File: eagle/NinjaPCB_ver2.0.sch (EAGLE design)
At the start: 76 parts, among them IC2 VNH3SP30-BNC, IC3 ANALOGSW_AD_SOT23-6NC, IC4 ANALOGSW_TI-SC70-5/6NC, IC5 MCP3551SNNC, IC6 NAU7802NC, J2 ATX24, J3 HEATER, J4 HEATER_TEMP, J5 PELTIER, Q2 IRF520NPBF, Q3 IRF520NPBF, U1 CJT1117-3.3-SOT223

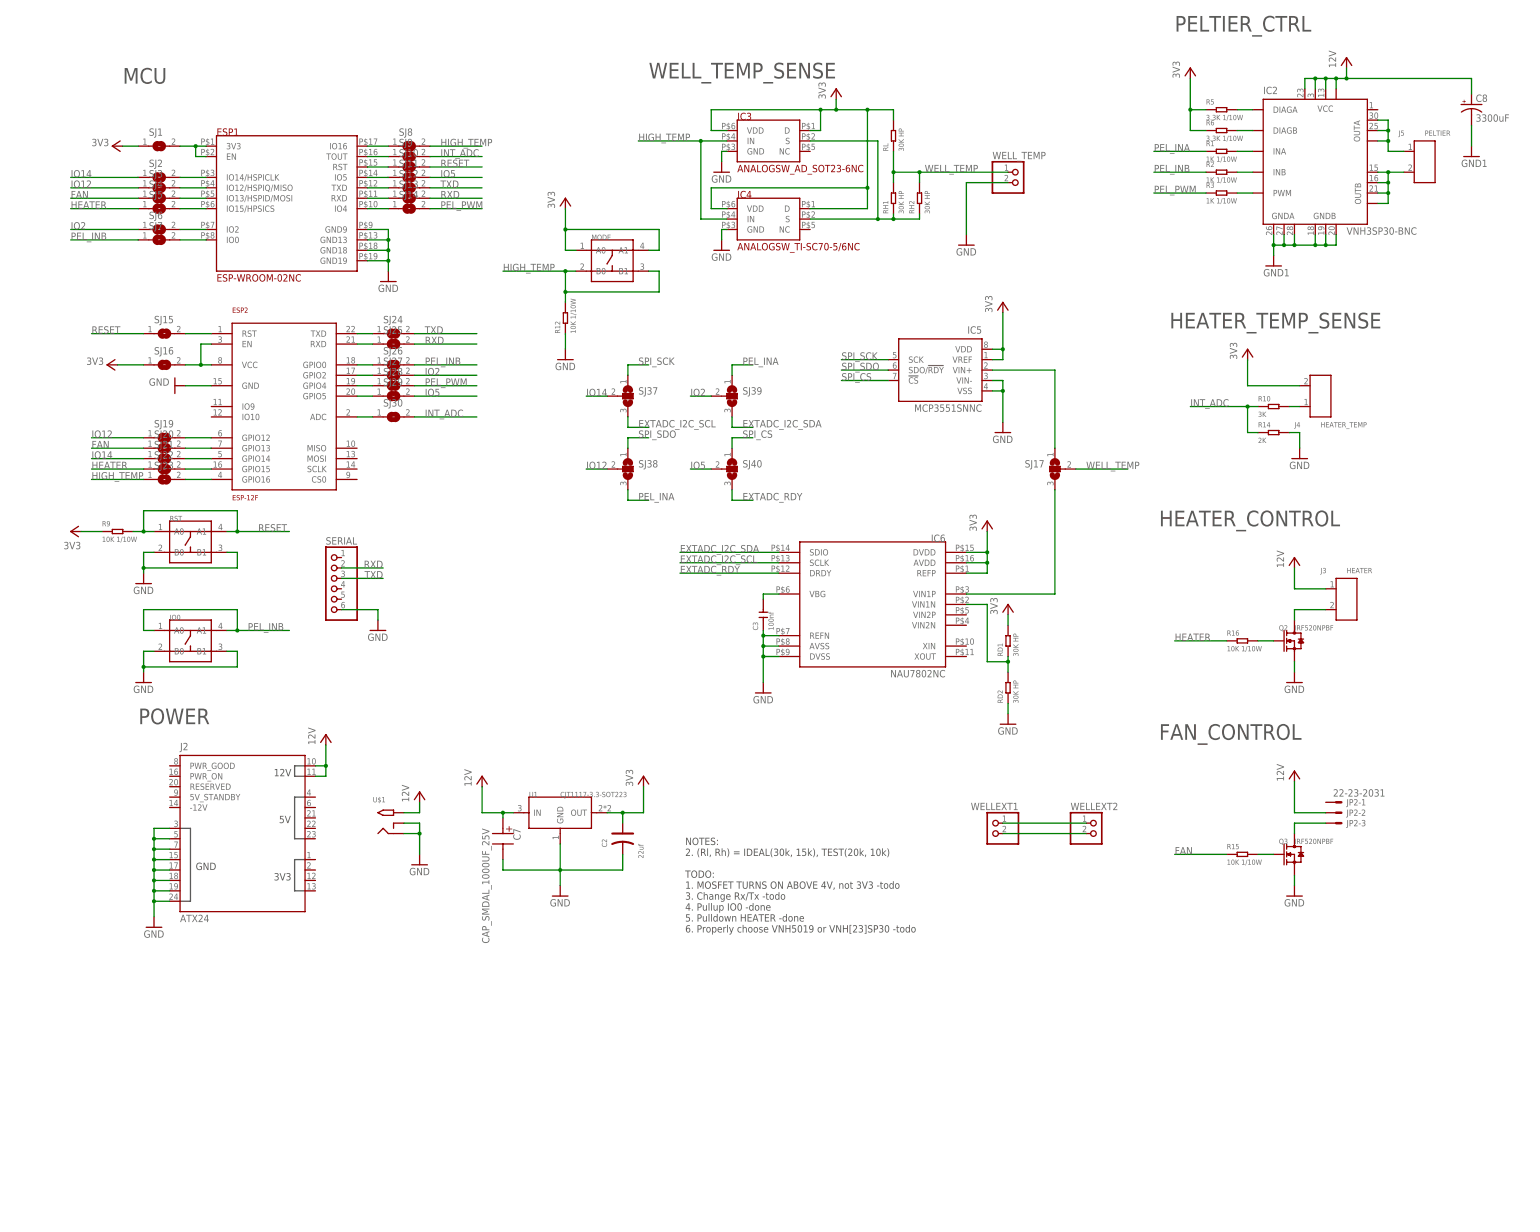
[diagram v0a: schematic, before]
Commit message: set default 4x4
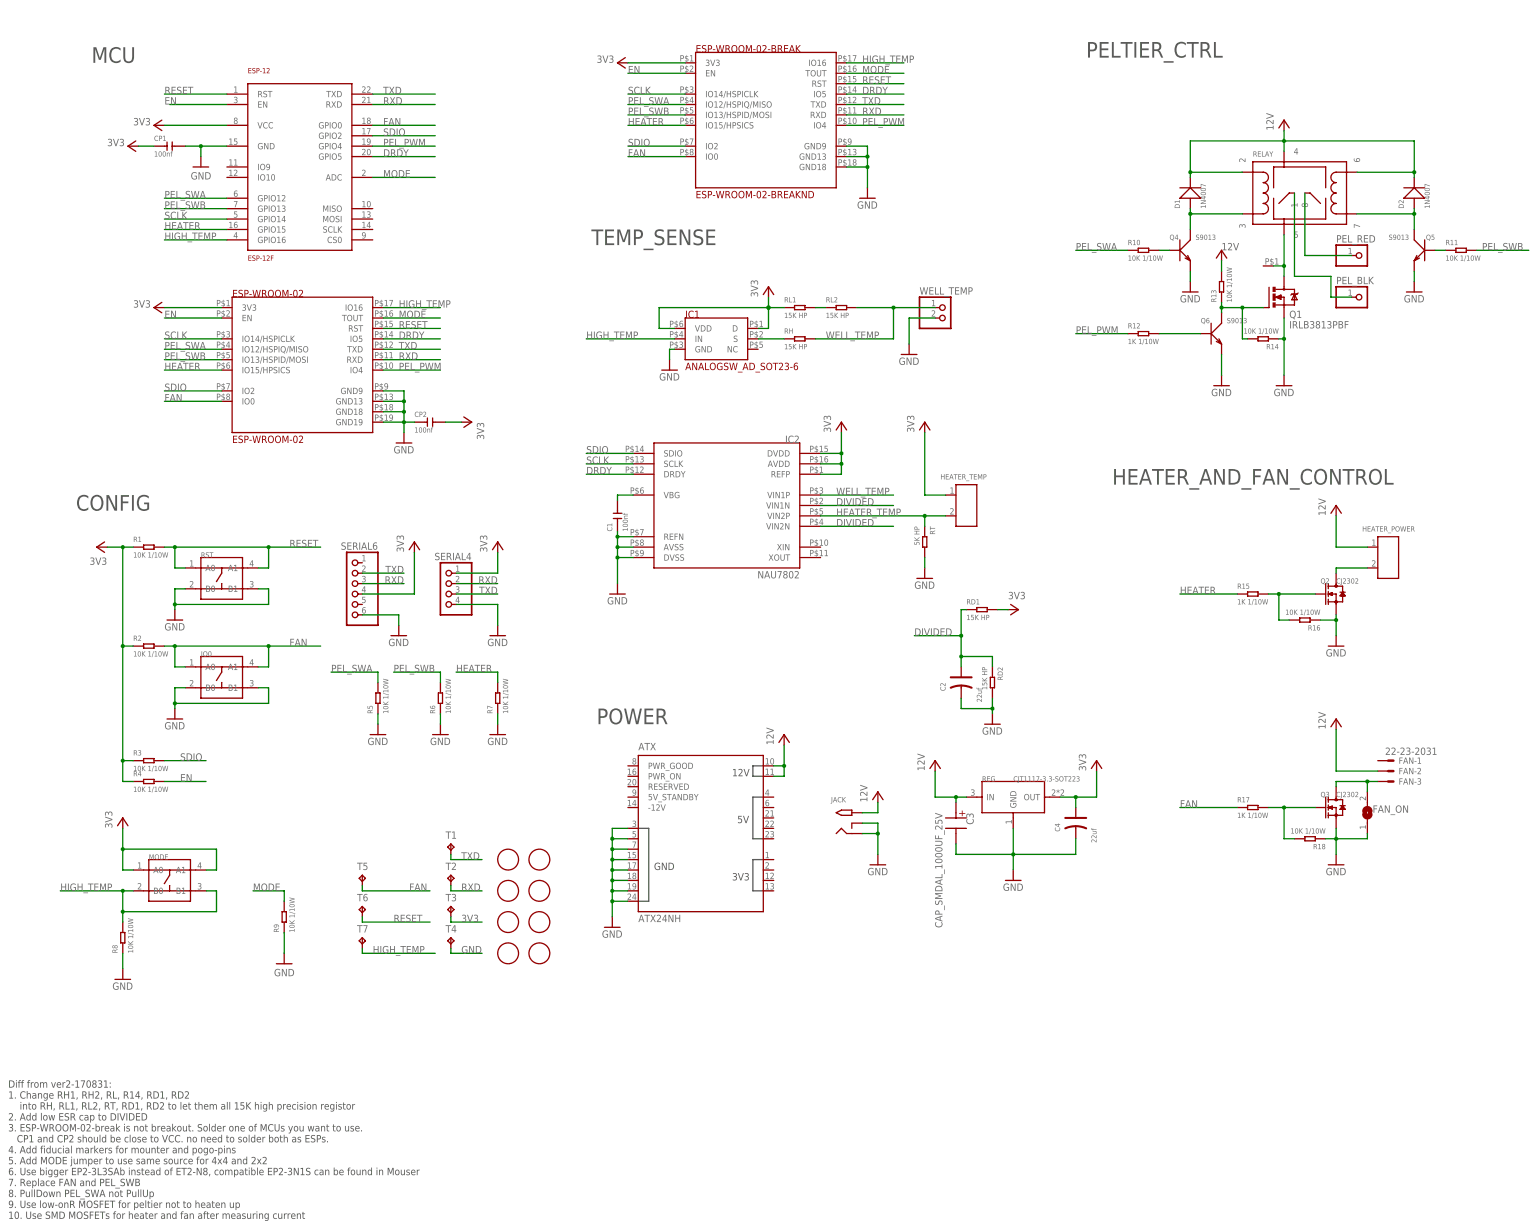
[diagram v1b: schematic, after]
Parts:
- removed C7: CAP_SMDAL_1000UF_25V, Seeed-OPL-2017-01-Capacitor-akita:CAP_SMDAL_1000UF_25V
- removed C8: 3300uF, PCR-RCL:CAP_E5-13-L3030RINV
- removed ESP1: ESP-WROOM-02NC, PCR-Module:ESP-WROOM-02NC
- removed ESP2: ESP-12F, Seeed-OPL-2017-01-Sensor-camilo:ESP-12F
- removed IC3: ANALOGSW_AD_SOT23-6NC, PCR-IC:ANALOGSW_AD_SOT23-6NC
- removed IC4: ANALOGSW_TI-SC70-5/6NC, PCR-IC:ANALOGSW_TI-SC70-5/6NC
- removed IC5: MCP3551SNNC, microchip:MCP3551SNNC
- removed IC6: NAU7802NC, PCR-IC:NAU7802NC
- removed J2: ATX24, PCR-Connector:ATX24
- removed J3: HEATER, Seeed-Connector:SCREW-TERMINAL-GREEN(2P-3.5)
- removed J4: HEATER_TEMP, Seeed-Connector:SCREW-TERMINAL-GREEN(2P-3.5)
- removed J5: PELTIER, Seeed-Connector:SCREW-TERMINAL-GREEN(2P-3.5)
- removed JP2: 22-23-2031, con-molex:22-23-2031
- removed RH1, RH2, RL: 30K HP, PCR-RCL:R0603NC
- removed SERIAL: (no value), pinhead:PINHD-1X6
- removed SJ1, SJ10, SJ11, SJ12, SJ13, SJ14, SJ15, SJ16, SJ19, SJ2, SJ20, SJ21, SJ22, SJ23, SJ24, SJ25, SJ26, SJ27, SJ28, SJ29, SJ3, SJ30, SJ4, SJ5, SJ6, SJ7, SJ8, SJ9: (no value), jumper:SJ
- removed SJ17, SJ37, SJ38, SJ39, SJ40: (no value), jumper:SJ2W
- removed U$1: 2.1MMJACKTHM, adafruit:2.1MMJACKTHM
- removed U1: CJT1117-3.3-SOT223, Seeed-IC:PMIC-CJT1117-3.3(SOT223)
- removed WELLEXT1, WELLEXT2: (no value), pinhead:PINHD-1X2
- added ATX: ATX24NH, PCR-Connector:ATX24NH
- added C1, CP1, CP2: 100nf, Seeed-Capacitor:CERAMIC-100NF-50V-10%-X7R(0603)
- added C4: 22uf, Seeed-Capacitor:TANTALUM-SMD-22UF-16V(AVX-B)
- added D1, D2: 1N4007, Seeed-Diode:DIODE-GEN-PURPOSE-1KV-1A(DO-214AC)
- added ESP-12: ESP-12F, Seeed-OPL-2017-01-Sensor-camilo:ESP-12F
- added ESP-WROOM-02: ESP-WROOM-02, PCR-Module:ESP-WROOM-02
- added ESP-WROOM-02-BREAK: ESP-WROOM-02-BREAKND, PCR-Module:ESP-WROOM-02-BREAKND
- added FAN: 22-23-2031, con-molex:22-23-2031
- added FAN_ON: (no value), jumper:SJ
- added HEATER_POWER, HEATER_TEMP: (no value), Seeed-Connector:SCREW-TERMINAL-GREEN(2P-3.5)
- added HEATSINK: HEAT111PB015, PCR-Connector:HEAT111PB015
- added IC1: ANALOGSW_AD_SOT23-6, PCR-IC:ANALOGSW_AD_SOT23-6
- added JACK: 2.1MMJACKTHM-NOOUT, adafruit:2.1MMJACKTHM-NOOUT
- added PEL_BLK, PEL_RED: (no value), pinhead:PINHD-1X1L
- added Q1: IRLB3813PBF, transistor-power:IRF520
- added Q4, Q5, Q6: S9013, Seeed-Transistor:SMD-TRANSISTORS-NPN-25V-500MA-S9013(SOT-23)
- added R11, R13, R18, R4, R7, R8: 10K 1/10W, Seeed-Resistor:SMD-RES-10K-5%-1/10W(0603)
- added R17: 1K 1/10W, Seeed-Resistor:SMD-RES-1K-5%-1/10W(0603)
- added REG: CJT1117-3.3-SOT223, Seeed-IC:PMIC-CJT1117-3.3(SOT223)
- added RELAY: NEC-RELAY2EP2, PCR-Switch:NEC-RELAY2EP2
- added RH, RL1, RL2: 15K HP, PCR-RCL:R0603
- added RT: 5K HP, Seeed-Resistor:SMD-RES-2K-1%-1/10W(0603)
- added SERIAL4: (no value), pinhead:PINHD-1X4
- added SERIAL6: (no value), pinhead:PINHD-1X6
- added T1, T2, T3, T4, T5, T6, T7: TPTP20R, testpad:TPTP20R
- added U$10, U$3, U$4, U$5, U$6, U$7, U$8, U$9: FIDUCIAL, adafruit:FIDUCIAL
- C3: value 100nf -> CAP_SMDAL_1000UF_25V; device Seeed-Capacitor:CERAMIC-100NF-50V-10%-X7R(0603) -> Seeed-OPL-2017-01-Capacitor-akita:CAP_SMDAL_1000UF_25V
- IC2: value VNH3SP30-BNC -> NAU7802; device st-microelectronics:VNH3SP30-BNC -> PCR-IC:NAU7802
- Q2, Q3: value IRF520NPBF -> CJ2302; device Seeed-Transistor:DIP-MOSFET-N-CH-100V-9.7A-IRF520NPBF(TO-220AB) -> Seeed-Transistor:SMD-MOSFET-N-CH-20V-2.1A-CJ2302(SOT-23)
- R1, R2, R3: value 1K 1/10W -> 10K 1/10W; device Seeed-Resistor:SMD-RES-1K-5%-1/10W(0603) -> Seeed-Resistor:SMD-RES-10K-5%-1/10W(0603)
- R10: value 3K -> 10K 1/10W; device Seeed-Resistor:SMD-RES-3K-1%-1/10W(0603) -> Seeed-Resistor:SMD-RES-10K-5%-1/10W(0603)
- R12, R15: value 10K 1/10W -> 1K 1/10W; device Seeed-Resistor:SMD-RES-10K-5%-1/10W(0603) -> Seeed-Resistor:SMD-RES-1K-5%-1/10W(0603)
- R14: value 2K -> 10K 1/10W; device Seeed-Resistor:SMD-RES-2K-1%-1/10W(0603) -> Seeed-Resistor:SMD-RES-10K-5%-1/10W(0603)
- R5, R6: value 3.3K 1/10W -> 10K 1/10W; device Seeed-Resistor:SMD-RES-3.3K-5%-1/10W(0603) -> Seeed-Resistor:SMD-RES-10K-5%-1/10W(0603)
- RD1, RD2: value 30K HP -> 15K HP; device PCR-RCL:R0603NC -> PCR-RCL:R0603
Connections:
- removed net EXTADC_I2C_SCL: IC6.SCLK, SJ37.3
- removed net EXTADC_I2C_SDA: IC6.SDIO, SJ39.3
- removed net EXTADC_RDY: IC6.DRDY, SJ40.3
- removed net I2C_WELL_TEMP: IC6.VIN1P, SJ17.3
- removed net INT_ADC: R10.1, R14.1, SJ30.2, SJ9.2
- removed net IO12: SJ19.1, SJ3.1, SJ38.2
- removed net IO14: SJ2.1, SJ21.1, SJ37.2
- removed net IO2: SJ27.2, SJ39.2, SJ6.1
- removed net IO5: SJ11.2, SJ29.2, SJ40.2
- removed net N$10: IC2.PWM, R3.2
- removed net N$11: ESP1.3V3, ESP1.EN, SJ1.2
- removed net N$12: ESP1.IO14/HSPICLK, SJ2.2
- removed net N$13: ESP1.IO12/HSPIQ/MISO, SJ3.2
- removed net N$14: ESP1.IO13/HSPID/MOSI, SJ4.2
- removed net N$15: ESP1.IO15/HPSICS, SJ5.2
- removed net N$16: ESP1.IO2, SJ6.2
- removed net N$17: ESP1.IO0, SJ7.2
- removed net N$18: ESP1.IO16, SJ8.1
- removed net N$19: ESP1.TOUT, SJ9.1
- removed net N$20: ESP1.RST, SJ10.1
- removed net N$21: ESP1.IO5, SJ11.1
- removed net N$22: ESP1.TXD, SJ12.1
- removed net N$23: ESP1.RXD, SJ13.1
- removed net N$24: ESP1.IO4, SJ14.1
- removed net N$26: WELLEXT1.1, WELLEXT2.1
- removed net N$28: WELLEXT1.2, WELLEXT2.2
- removed net N$40: ESP2.RST, SJ15.2
- removed net N$42: ESP2.EN, ESP2.VCC, SJ16.2
- removed net N$43: ESP2.TXD, SJ24.1
- removed net N$44: ESP2.RXD, SJ25.1
- removed net N$45: ESP2.GPIO0, SJ26.1
- removed net N$46: ESP2.GPIO2, SJ27.1
- removed net N$47: ESP2.GPIO4, SJ28.1
- removed net N$48: ESP2.GPIO5, SJ29.1
- removed net N$49: ESP2.ADC, SJ30.1
- removed net N$67: ESP2.GPIO12, SJ19.2
- removed net N$68: ESP2.GPIO13, SJ20.2
- removed net N$69: ESP2.GPIO14, SJ21.2
- removed net N$70: ESP2.GPIO15, SJ22.2
- removed net N$71: ESP2.GPIO16, SJ23.2
- removed net N$9: IC2.INB, R2.2
- removed net N$91: IC6.VIN1N, RD1.1, RD2.2
- removed net OUTA: IC2.OUTA@1, IC2.OUTA@2, IC2.OUTA@3, J5.1
- removed net OUTB: IC2.OUTB, IC2.OUTB@1, IC2.OUTB@2, IC2.OUTB@3, J5.2
- removed net PEL_INA: R1.1, SJ38.3, SJ39.1
- removed net PEL_INB: IO0.A0, IO0.A1, R2.1, SJ26.2, SJ7.1
- removed net SPI_CS: IC5.!CS, SJ40.1
- removed net SPI_SCK: IC5.SCK, SJ37.1
- removed net SPI_SDO: IC5.SDO/!RDY, SJ38.1
- removed net SPI_WELL_TEMP: IC5.VIN+, SJ17.1
- new net DIVIDED: C2.+, IC2.VIN1N, IC2.VIN2N, RD1.1, RD2.1
- new net DRDY: ESP-12.GPIO5, ESP-WROOM-02-BREAK.IO5, ESP-WROOM-02.IO5, IC2.DRDY
- new net EN: ESP-12.EN, ESP-WROOM-02-BREAK.EN, ESP-WROOM-02.EN, R4.2
- new net HEATER_TEMP: HEATER_TEMP.2, IC2.VIN2P, RT.1
- new net MODE: ESP-12.ADC, ESP-WROOM-02-BREAK.TOUT, ESP-WROOM-02.TOUT, R9.2
- new net N$30: Q6.B, R12.2
- new net N$32: Q2.G, R15.2, R16.2
- new net N$33: D1.+, Q4.C, RELAY.3
- new net N$34: Q4.B, R10.2
- new net N$35: Q5.B, R11.1
- new net N$36: D2.+, Q5.C, RELAY.7
- new net PEL_SWA: ESP-12.GPIO12, ESP-WROOM-02-BREAK.IO12/HSPIQ/MISO, ESP-WROOM-02.IO12/HSPIQ/MISO, R10.1, R5.2
- new net PEL_SWB: ESP-12.GPIO13, ESP-WROOM-02-BREAK.IO13/HSPID/MOSI, ESP-WROOM-02.IO13/HSPID/MOSI, R11.2, R6.2
- new net SCLK: ESP-12.GPIO14, ESP-WROOM-02-BREAK.IO14/HSPICLK, ESP-WROOM-02.IO14/HSPICLK, IC2.SCLK
- new net SDIO: ESP-12.GPIO2, ESP-WROOM-02-BREAK.IO2, ESP-WROOM-02.IO2, IC2.SDIO, R3.2
- net 12V: now also ATX.12V_10, ATX.12V_11, C3.P$P, D1.-, D2.-, FAN-2.S, HEATER_POWER.1, JACK.TIP, R13.2, REG.IN, RELAY.2, RELAY.4, RELAY.6; no longer C7.P$P, C8.+, IC2.VCC, IC2.VCC@1, IC2.VCC@2, IC2.VCC@3, J2.12V_10, J2.12V_11, J3.1, JP2-2.S, U$1.TIP, U1.IN
- net 3V3: now also C4.+, CP1.1, CP2.2, ESP-12.VCC, ESP-WROOM-02-BREAK.3V3, ESP-WROOM-02.3V3, HEATER_TEMP.1, IC1.D, IC1.VDD, IC2.AVDD, IC2.DVDD, IC2.REFP, R1.1, R2.1, R3.1, R4.1, REG.OUT, RL1.1, SERIAL4.1, SERIAL6.4, T3.TP; no longer C2.+, IC3.D, IC3.VDD, IC4.D, IC4.VDD, IC5.VDD, IC5.VREF, IC6.AVDD, IC6.DVDD, IC6.REFP, J4.2, R5.1, R6.1, R9.1, RL.2, SJ1.1, SJ16.1, U1.OUT
- net FAN: now also ESP-12.GPIO0, ESP-WROOM-02-BREAK.IO0, ESP-WROOM-02.IO0, IO0.A0, IO0.A1, R17.1, R2.2, T5.TP; no longer R15.1, SJ20.1, SJ4.1
- net GND: now also ATX.GND15, ATX.GND17, ATX.GND18, ATX.GND19, ATX.GND24, ATX.GND3, ATX.GND5, ATX.GND7, C1.1, C3.P$M, C4.-, CP1.2, CP2.1, ESP-12.GND, ESP-WROOM-02-BREAK.GND13, ESP-WROOM-02-BREAK.GND18, ESP-WROOM-02-BREAK.GND9, ESP-WROOM-02.GND13, ESP-WROOM-02.GND18, ESP-WROOM-02.GND19, ESP-WROOM-02.GND9, FAN_ON.1, IC1.GND, IC2.AVSS, IC2.DVSS, IC2.REFN, JACK.RING, JACK.RING_SW, Q1.S, Q4.E, Q5.E, Q6.E, R14.1, R16.1, R18.1, R5.1, R6.1, R7.1, R8.1, R9.1, RD2.2, REG.GND, RT.2, SERIAL4.4, SERIAL6.6, T4.TP; no longer C3.1, C7.P$M, C8.-, ESP1.GND13, ESP1.GND18, ESP1.GND19, ESP1.GND9, ESP2.GND, IC2.GNDA, IC2.GNDA@1, IC2.GNDA@2, IC2.GNDB, IC2.GNDB@1, IC2.GNDB@2, IC3.GND, IC4.GND, IC5.VIN-, IC5.VSS, IC6.AVSS, IC6.DVSS, IC6.REFN, J2.GND15, J2.GND17, J2.GND18, J2.GND19, J2.GND24, J2.GND3, J2.GND5, J2.GND7, R12.1, R14.2, RD2.1, SERIAL.6, U$1.RING, U$1.RING_SW, U1.GND
- net HEATER: now also ESP-12.GPIO15, ESP-WROOM-02-BREAK.IO15/HPSICS, ESP-WROOM-02.IO15/HPSICS, R15.1, R7.2; no longer R16.1, SJ22.1, SJ5.1
- net HIGH_TEMP: now also ESP-12.GPIO16, ESP-WROOM-02-BREAK.IO16, ESP-WROOM-02.IO16, IC1.IN, R8.2, T7.TP; no longer IC3.IN, IC4.IN, R12.2, SJ23.1, SJ8.2
- net N$1: now also RL1.2, RL2.1; no longer J4.1, R10.2
- net N$2: now also HEATER_POWER.2; no longer J3.2
- net N$27: now also IC1.S, RH.1; no longer IC3.S, IC4.S, RH1.1, RH2.1
- net N$3: now also HEATSINK.P$1, Q1.D, RELAY.5; no longer Q2.G, R16.2
- net N$4: now also FAN-3.S, FAN_ON.2; no longer JP2-3.S
- net N$5: now also Q1.G, Q6.C, R13.1, R14.2; no longer Q3.G, R15.2
- net N$6: now also PEL_RED.1, RELAY.8; no longer IC2.DIAGA, R5.2
- net N$7: now also PEL_BLK.1, RELAY.1; no longer IC2.DIAGB, R6.2
- net N$8: now also Q3.G, R17.2, R18.2; no longer IC2.INA, R1.2
- net N$92: now also C1.2, IC2.VBG; no longer C3.2, IC6.VBG
- net PEL_PWM: now also ESP-12.GPIO4, ESP-WROOM-02-BREAK.IO4, ESP-WROOM-02.IO4, R12.1; no longer R3.1, SJ14.2, SJ28.2
- net RESET: now also ESP-12.RST, ESP-WROOM-02-BREAK.RST, ESP-WROOM-02.RST, R1.2, T6.TP; no longer R9.2, SJ10.2, SJ15.1
- net RXD: now also ESP-12.RXD, ESP-WROOM-02-BREAK.RXD, ESP-WROOM-02.RXD, SERIAL4.2, SERIAL6.3, T2.TP; no longer SERIAL.2, SJ13.2, SJ25.2
- net TXD: now also ESP-12.TXD, ESP-WROOM-02-BREAK.TXD, ESP-WROOM-02.TXD, SERIAL4.3, SERIAL6.2, T1.TP; no longer SERIAL.3, SJ12.2, SJ24.2
- net WELL_TEMP: now also IC2.VIN1P, RH.2, RL2.2; no longer RH1.2, RH2.2, RL.1, SJ17.2
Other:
- note added: "CONFIG"
- note added: "Diff from ver2-170831: 1. Change RH1, RH2, RL, R14, RD1, RD2 into RH, RL1, RL2, RT, RD1, RD2 to let them all 15K high precision registor 2. Add low ESR cap to DIVIDED 3. ESP-WROOM-02-break is not breakout. Solder one of MCUs you want to use. CP1 and CP2 should be close to VCC. no need to solder both as ESPs. 4. Add fiducial markers for mounter and pogo-pins 5. Add MODE jumper to use same source f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"
- note added: "HEATER_AND_FAN_CONTROL"
- note added: "TEMP_SENSE"
- note removed: "FAN_CONTROL"
- note removed: "HEATER_CONTROL"
- note removed: "HEATER_TEMP_SENSE"
- note removed: "NOTES: 2. (Rl, Rh) = IDEAL(30k, 15k), TEST(20k, 10k) TODO: 1. MOSFET TURNS ON ABOVE 4V, not 3V3 -todo 3. Change Rx/Tx -todo 4. Pullup IO0 -done 5. Pulldown HEATER -done 6. Properly choose VNH5019 or VNH[23]SP30 -todo"
- note removed: "WELL_TEMP_SENSE"
- moved on the sheet: C2, IC2, IO0, MODE, Q2, Q3, R1, R10, R12, R14, R15, R16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

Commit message: remove wrong schematics
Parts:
- RELAY: value NEC-RELAY2EP2 -> NEC-RELAY2EN2; device PCR-Switch:NEC-RELAY2EP2 -> PCR-Switch:NEC-RELAY2EN2
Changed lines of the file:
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@@
 <part name="R13" library="Seeed-Resistor" deviceset="SMD-RES-10K-5%-1/10W(0603)" device="" value="10K 1/10W"/>
 <part name="R14" library="Seeed-Resistor" deviceset="SMD-RES-10K-5%-1/10W(0603)" device="" value="10K 1/10W"/>
-<part name="RELAY" library="PCR-Switch" deviceset="NEC-RELAY2" device="EP2" value="NEC-RELAY2EP2"/>
+<part name="RELAY" library="PCR-Switch" deviceset="NEC-RELAY2" device="EN2" value="NEC-RELAY2EN2"/>
 <part name="D1" library="Seeed-Diode" deviceset="DIODE-GEN-PURPOSE-1KV-1A(DO-214AC)" device="" value="1N4007"/>
 <part name="D2" library="Seeed-Diode" deviceset="DIODE-GEN-PURPOSE-1KV-1A(DO-214AC)" device="" value="1N4007"/>
